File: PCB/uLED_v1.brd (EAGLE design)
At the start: 160 x 100 mm, 17 parts, among them IC1 ATSAMD21E, J2 455-1750-1-ND, SW1 EG1218, U1 AP2112K-3.3

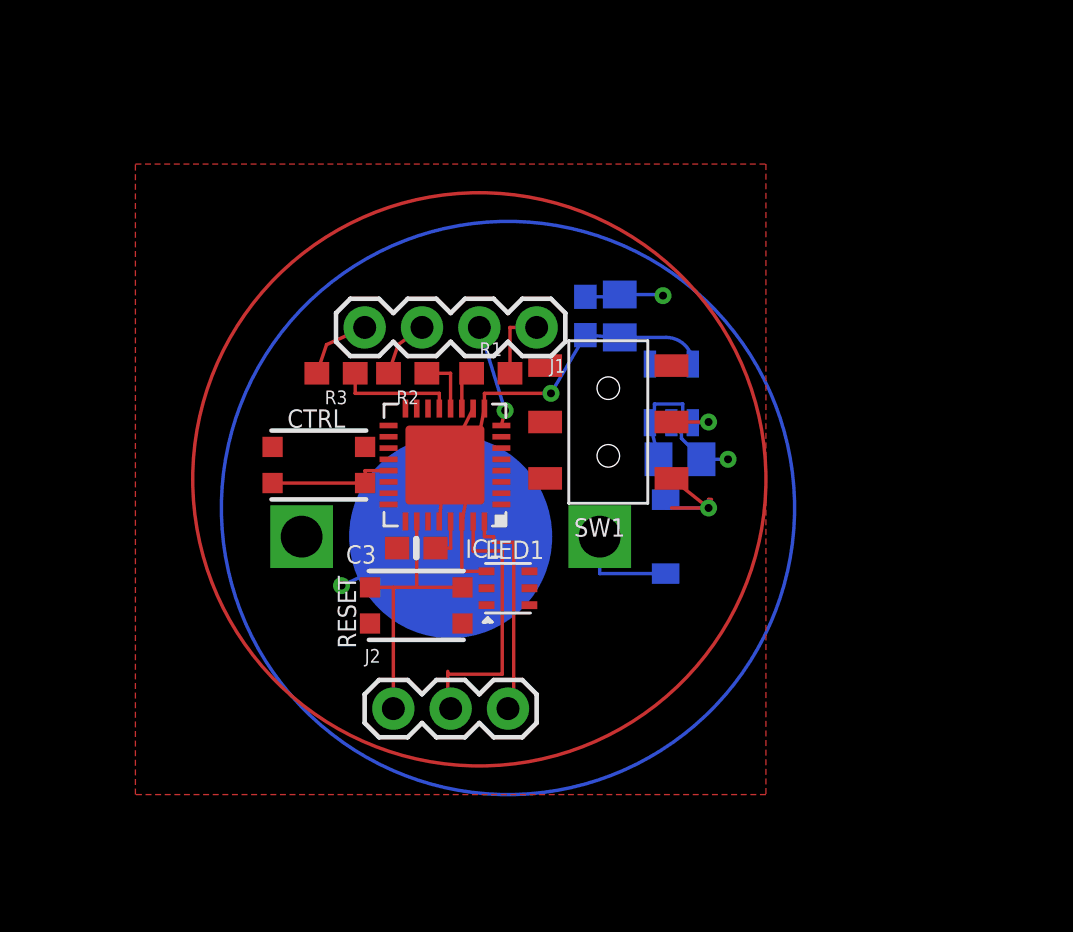
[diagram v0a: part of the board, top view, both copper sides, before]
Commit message: Updating board again
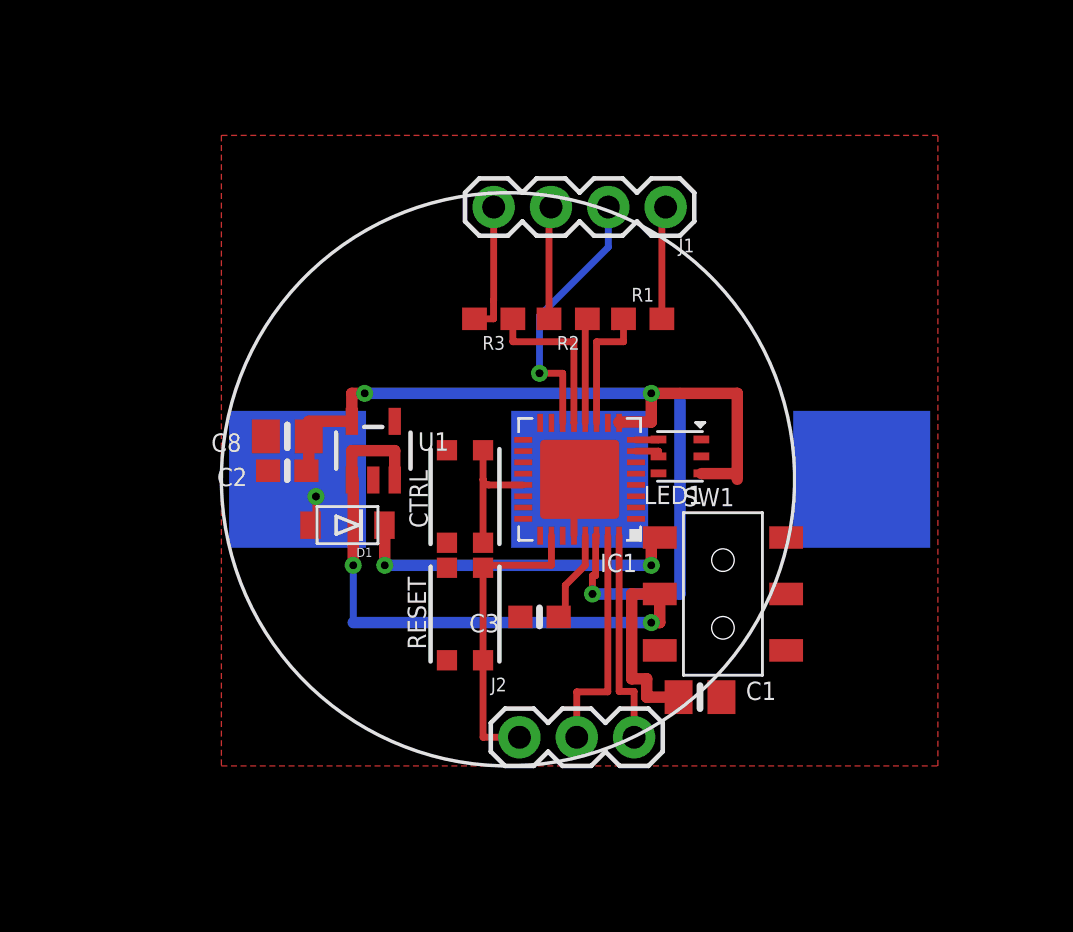
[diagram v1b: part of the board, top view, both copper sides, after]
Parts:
- removed BT1: (no value), SparkFun-Batteries:BATTCON_12MM_PTH
- added BT2: (no value), SparkFun-Batteries:BATTCON_20MM
- moved C8 15.7 mm to (35.9, 26.0), flipped to the top, turned to 180 degrees
- moved C2 14.9 mm to (35.9, 24.5), flipped to the top, turned to 180 degrees
- moved D1 14.1 mm to (38.6, 22.1), flipped to the top, turned to 180 degrees
- moved U1 13.5 mm to (39.8, 25.4), flipped to the top
- moved C1 10.6 mm to (54.2, 14.5), flipped to the top, turned to 0 degrees
- moved LED1 9.60 mm to (53.3, 25.1), turned to 180 degrees
- moved SW1 9.16 mm to (55.2, 19.1), turned to 270 degrees
- moved J1 7.82 mm to (52.7, 36.2)
- moved R2 7.51 mm to (48.4, 31.2)
- moved R3 7.39 mm to (45.1, 31.2)
- moved R1 7.15 mm to (51.7, 31.2)
- moved CTRL 6.63 mm to (43.8, 23.4), turned to 270 degrees
- moved C3 6.25 mm to (47.1, 18.0)
- moved IC1 6.00 mm to (48.9, 24.1)
- moved J2 5.73 mm to (46.2, 12.7)
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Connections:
- new net LEDCI: IC1.7, LED1.5
- new net LEDDI: IC1.8, LED1.6
- net ANODE: now also IC1.14; no longer IC1.8
- net GND: now also BT2.2; no longer BT1.GND
- net VBAT: now also BT2.1; no longer BT1.VCC@1
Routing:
- net 3.3V: track 20.3 -> 47.4 mm, vias 1 -> 3
- net VOUT: track 7.57 -> 33.7 mm, vias 1 -> 2
- net GND: track 23.3 -> 2.75 mm, vias 3 -> 0
- net VHIGH: track 6.53 -> 15.2 mm, vias 1 -> 2
- net ANODE: track 4.54 -> 11.9 mm
- net REDOUT: track 1.74 -> 6.42 mm
- net N$2: track 3.19 -> 5.80 mm
- net N$3: track 2.64 -> 5.04 mm
- net VDDCORE: track 1.86 -> 4.26 mm
- net VBAT: track 4.56 -> 2.50 mm, vias 0 -> 1
- net GREENOUT: track 2.62 -> 4.65 mm
- net BLUEOUT: track 5.29 -> 7.32 mm
- net SWCLK: track 12.3 -> 10.3 mm
- net N$1: track 3.21 -> 5.12 mm
- net LEDCI: track 0.00 -> 1.23 mm
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
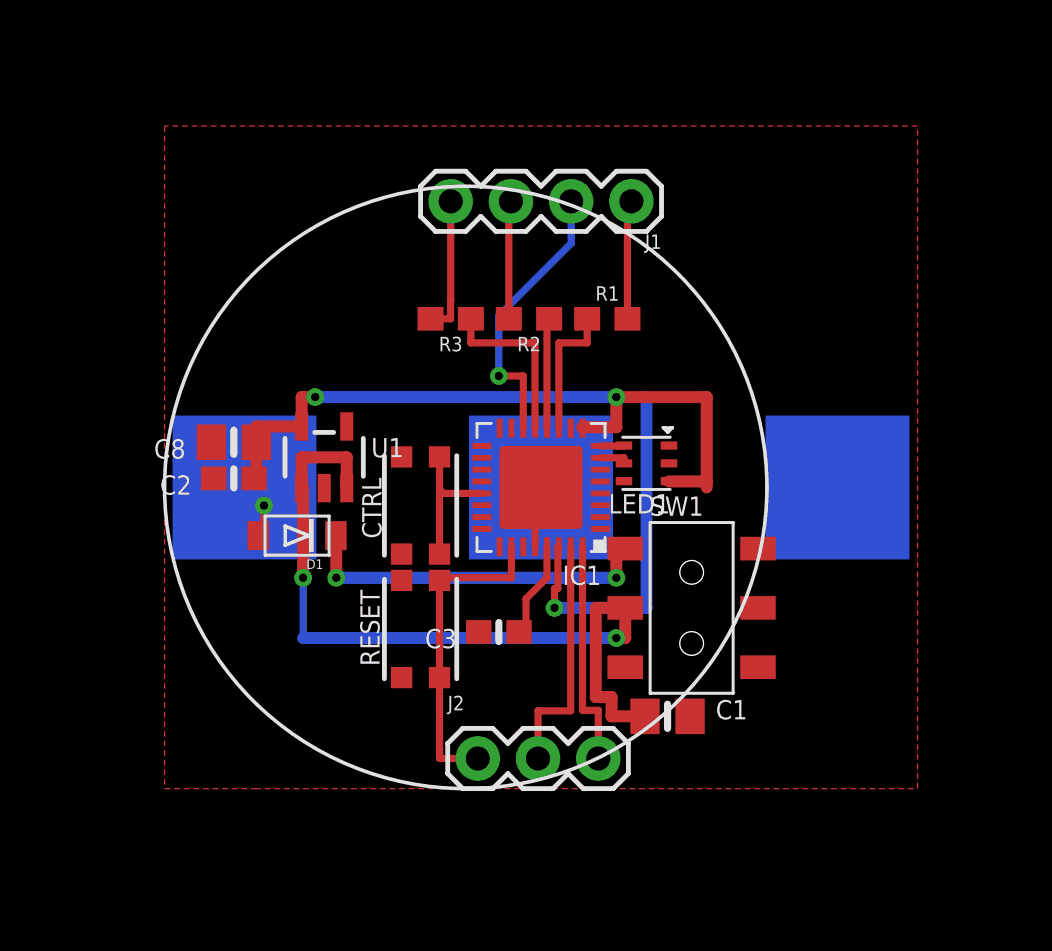
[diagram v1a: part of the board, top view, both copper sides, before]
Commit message: yet another pcb
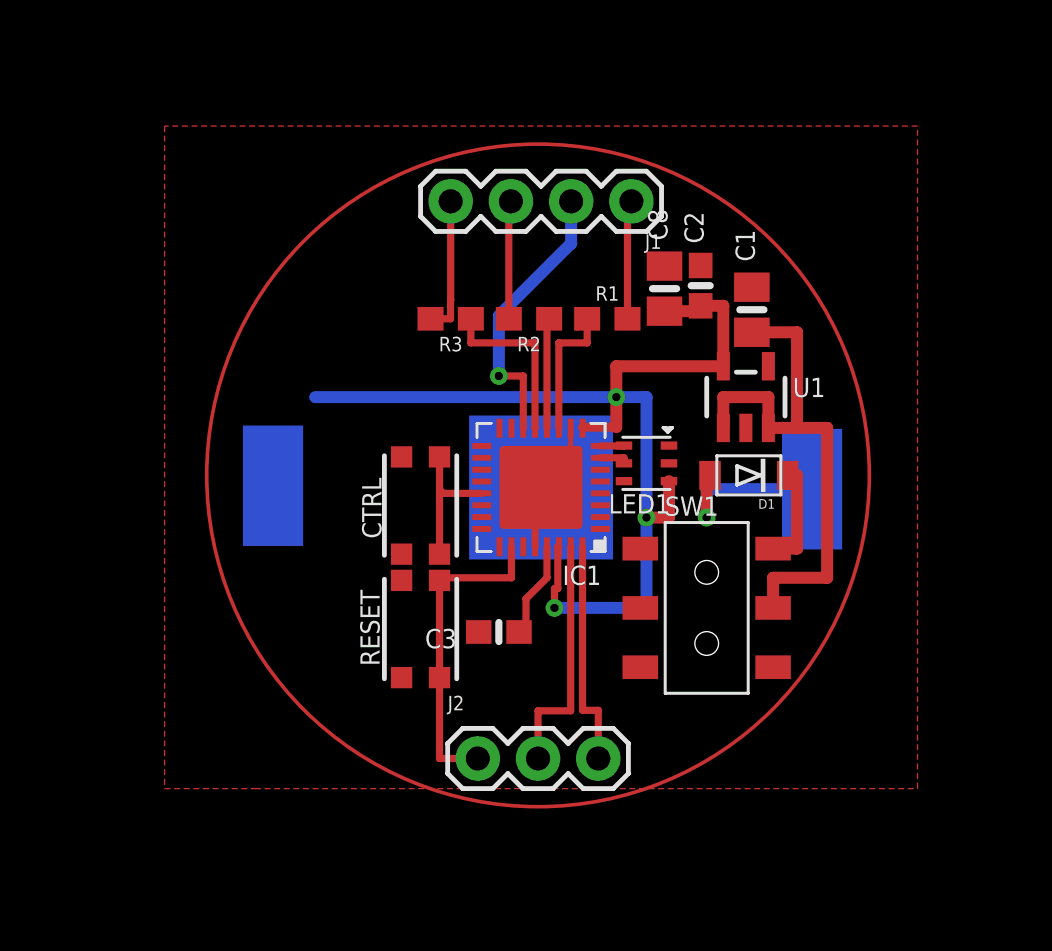
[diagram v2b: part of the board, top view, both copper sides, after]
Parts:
- removed BT2: (no value), SparkFun-Batteries:BATTCON_20MM
- added U$3: 20MM_BATTERY, mikes:BATTCON_20MM
- moved C2 21.3 mm to (55.6, 32.6), turned to 90 degrees
- moved C8 19.3 mm to (54.1, 32.5), turned to 90 degrees
- moved D1 19.2 mm to (57.7, 24.6)
- moved U1 18.0 mm to (57.5, 27.9)
- moved C1 17.5 mm to (57.8, 31.6), turned to 90 degrees
- moved SW1 0.64 mm to (55.9, 19.1)
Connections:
- new net +1: U$3.1
- net GND: now also U$3.2; no longer BT2.2
- net VBAT: now also U$3.3; no longer BT2.1
- net VHIGH: now also SW1.O1; no longer SW1.O2
- net VOUT: now also SW1.P1; no longer SW1.P2
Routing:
- net VOUT: track 33.7 -> 22.8 mm, vias 2 -> 0
- net VHIGH: track 15.2 -> 4.75 mm, vias 2 -> 0
- net VBAT: track 2.50 -> 7.56 mm
- net GND: track 2.75 -> 5.77 mm
- net 3.3V: track 47.4 -> 45.8 mm
